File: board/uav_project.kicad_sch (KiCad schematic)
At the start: 0 parts

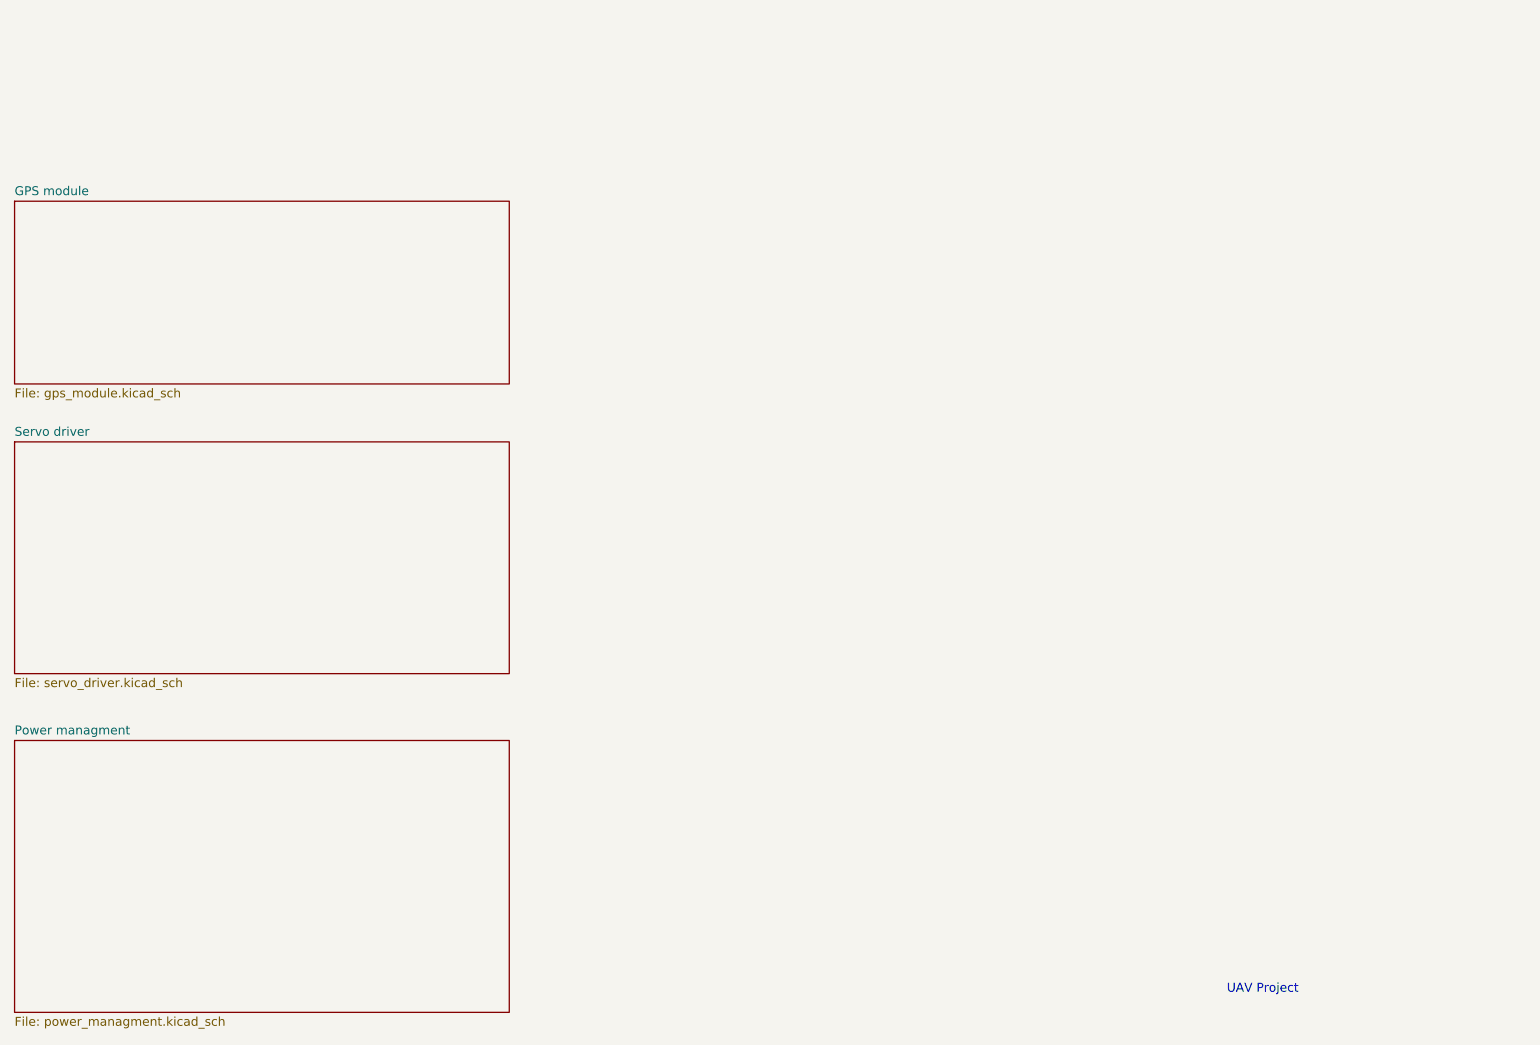
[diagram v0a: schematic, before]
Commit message: Hopefully finished schema for pcb
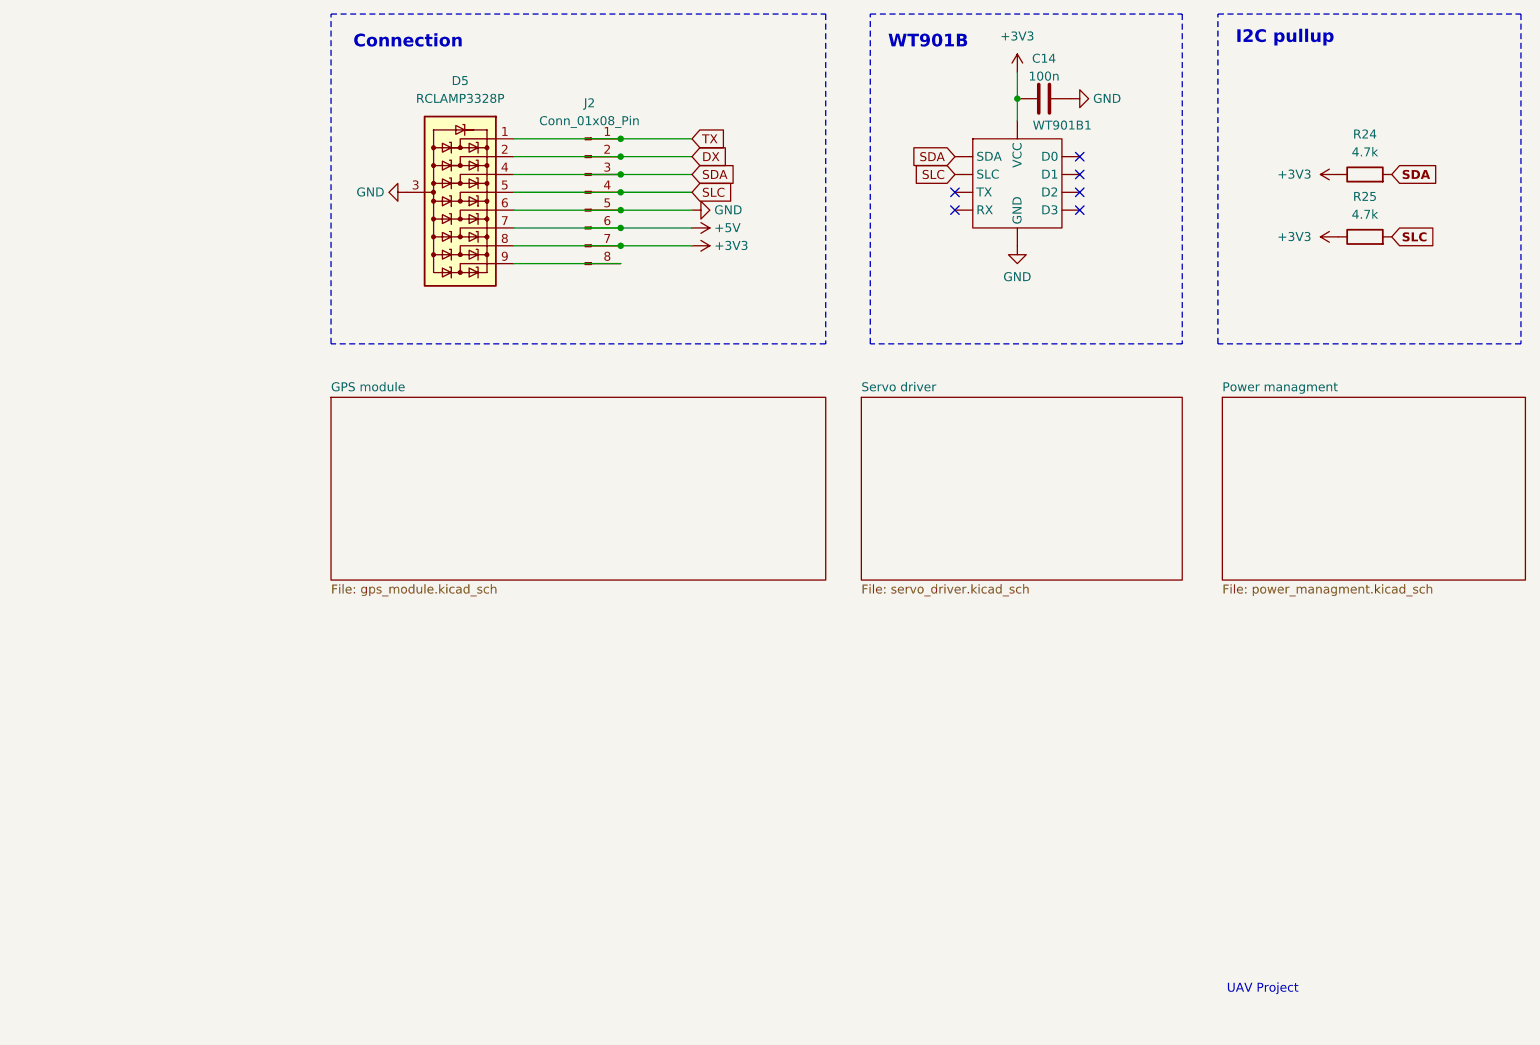
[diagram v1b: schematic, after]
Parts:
- added C14: 100n, symbol Device:C
- added D5: RCLAMP3328P, Package_DFN_QFN:UDFN-9_1.0x3.8mm_P0.5mm, symbol Power_Protection:RCLAMP3328P
- added J2: Conn_01x08_Pin, symbol Connector:Conn_01x08_Pin
- added R24, R25: 4.7k, symbol Device:R
- added WT901B1: ~, symbol .kicad_sym:WT901B
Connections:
- new net: D5.9 (K8), J2.8 (Pin_8)
- new net +3V3: C14.1, D5.8 (K7), J2.7 (Pin_7), R24.1, R25.1, WT901B1. (VCC)
- new net +5V: D5.7 (K6), J2.6 (Pin_6)
- new net DX: D5.2 (K2), J2.2 (Pin_2)
- new net GND: C14.2, D5.3 (A), D5.6 (K5), J2.5 (Pin_5), WT901B1. (VCC)
- new net SDA: D5.4 (K3), J2.3 (Pin_3), R24.2, WT901B1. (VCC)
- new net SLC: D5.5 (K4), J2.4 (Pin_4), R25.2, WT901B1. (VCC)
- new net TX: D5.1 (K1), J2.1 (Pin_1)
- no-connect marks 0 -> 6
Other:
- note added: "Connection"
- note added: "I2C pullup"
- note added: "WT901B"
